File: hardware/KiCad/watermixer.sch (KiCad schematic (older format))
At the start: 14 parts, among them U1 MCP4728

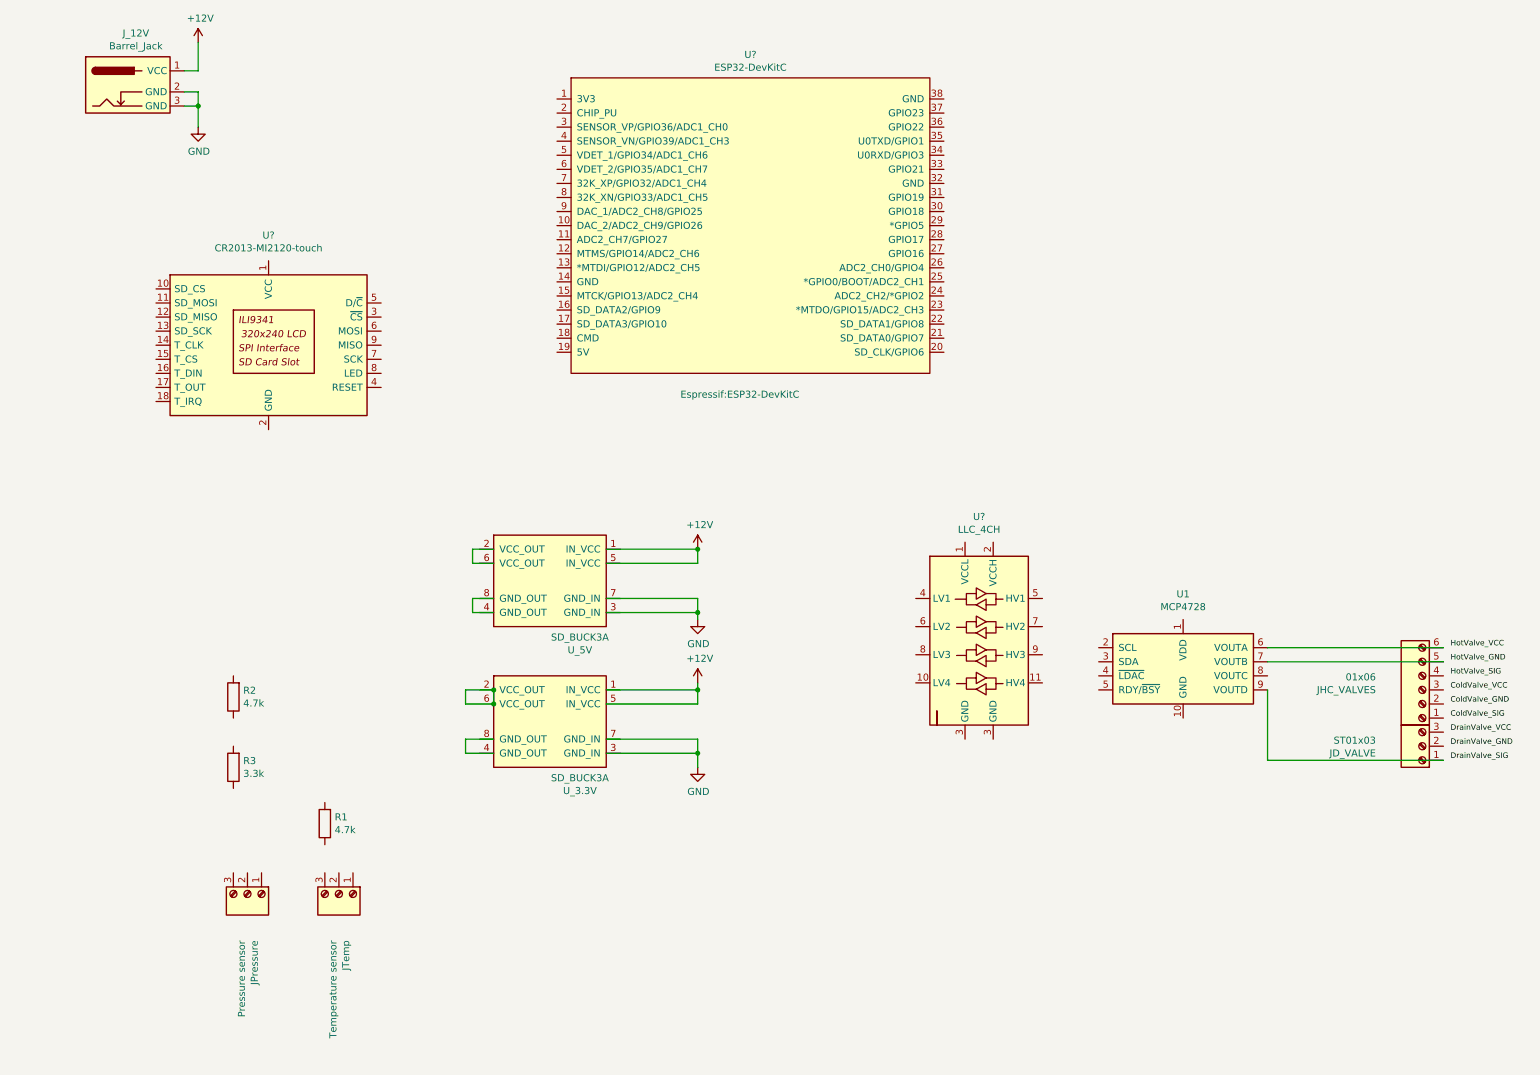
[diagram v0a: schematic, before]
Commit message: Done connecting all parts on the schema
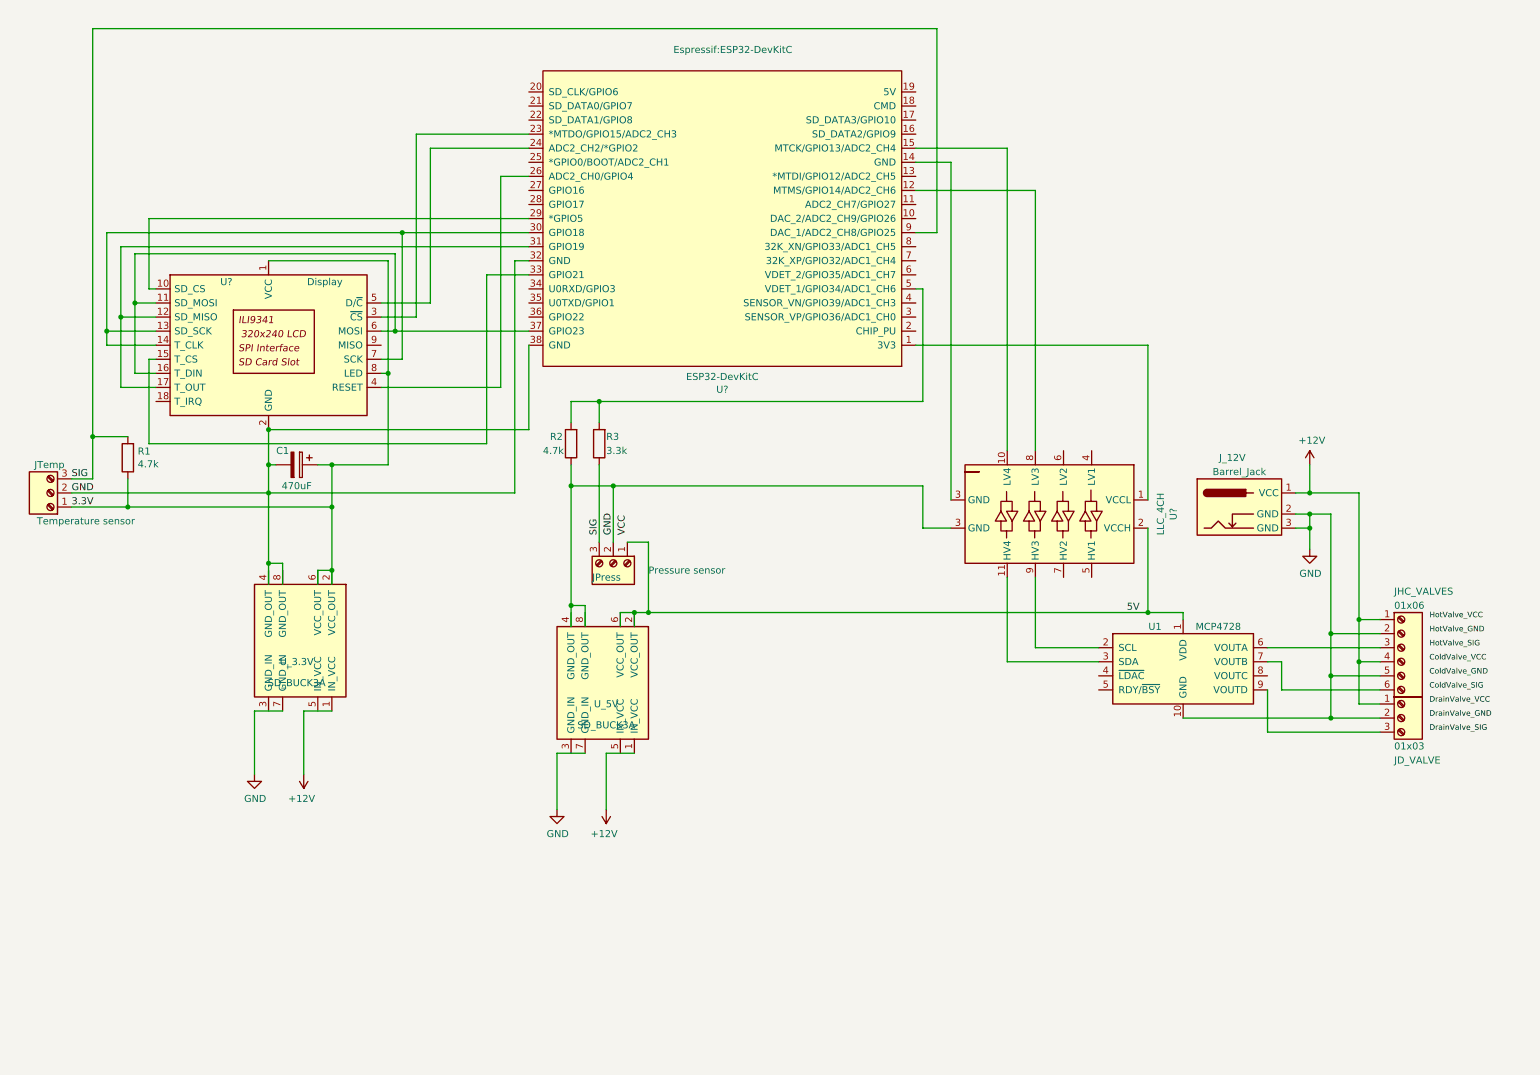
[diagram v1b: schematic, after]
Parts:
- removed U?: CR2013-MI2120-touch, Display:CR2013-MI2120, symbol watermixer-symbols:CR2013-MI2120-touch
- added C1: 470uF, Capacitor_THT:CP_Radial_Tantal_D8.0mm_P5.00mm, symbol watermixer-symbols:CP
- added U?: Display, watermixer-footprints:CR2013-MI2120_touch, symbol watermixer-symbols:CR2013-MI2120-touch
- JD_VALVE: value ST01x03 -> 01x03
- renumbered JPressure to JPress
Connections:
- net labels added: 3.3V, 5V, SIG, VCC
- wire segments 38 -> 146
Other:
- moved on the sheet: JD_VALVE, JHC_VALVES, JPress, JTemp, J_12V, R1, R2, R3, U?, U_3.3V, U_5V
